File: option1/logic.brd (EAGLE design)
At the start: 37.4 x 33 mm, 8 parts, among them CON1 PINHEAD_1X10-2, CON2 PINHEAD_1X10-2, CON4 PINHEAD_1X02-2, CON5 PINHEAD_1X02-2, CON6 PINHEAD_1X04-2

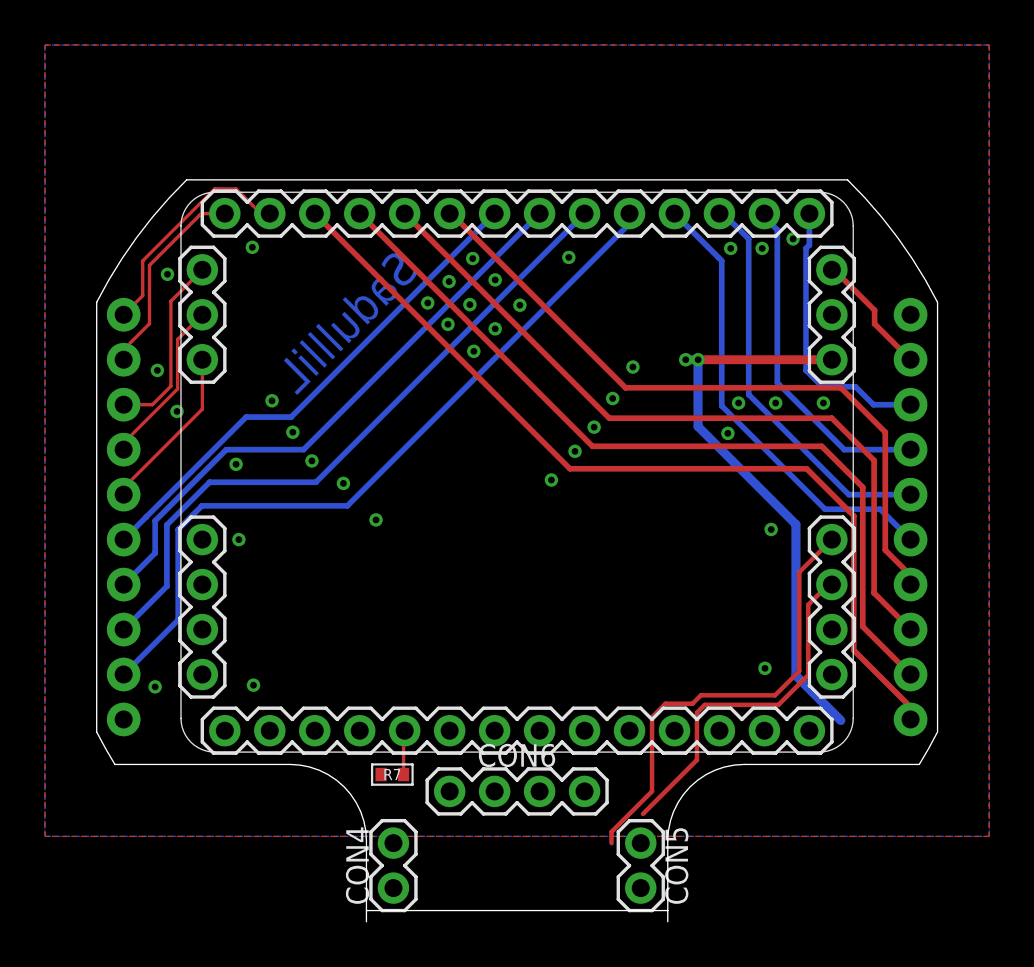
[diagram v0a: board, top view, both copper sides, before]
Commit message: updates here and there
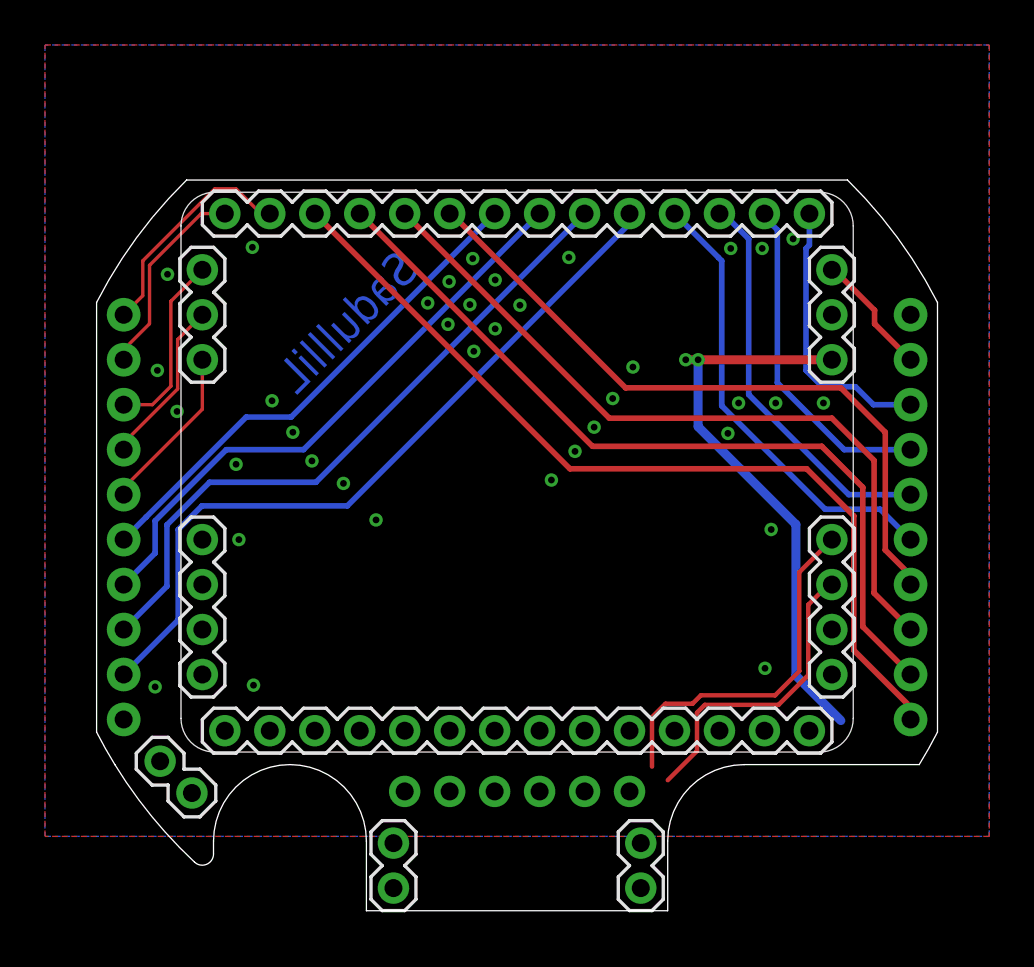
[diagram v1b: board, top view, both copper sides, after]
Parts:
- removed R7: 1K, R_digikey:R0402
- added CON3: PINHEAD_1X06-2, pinhead:1X06-PTH-2
- CON6: value PINHEAD_1X04-2 -> PINHEAD_1X02-2; device pinhead:1X04-PTH-2 -> pinhead:1X02-PTH-2
- moved CON6 15.2 mm to (-15.2, -11.6), turned to 135 degrees
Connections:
- removed net N$18: MODULE2.29, R7.1
- new net ADJ: MODULE2.29
- new net GPIO1: MODULE2.27
- new net GPIO2: MODULE2.28
- net GND: no longer R7.2
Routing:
- net CAN1_TX: track 20.2 -> 16.0 mm
- net N$18: track 1.97 -> 0.00 mm
- net CAN1_RX: track 15.7 -> 13.7 mm
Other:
- board size 37.4 x 33 mm -> 37.4 x 32.5 mm
